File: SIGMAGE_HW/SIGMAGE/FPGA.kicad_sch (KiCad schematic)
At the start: 52 parts, among them J9 TSW10607GS, U41 MMBT2222A, U8 LFE5U25F6BG256I

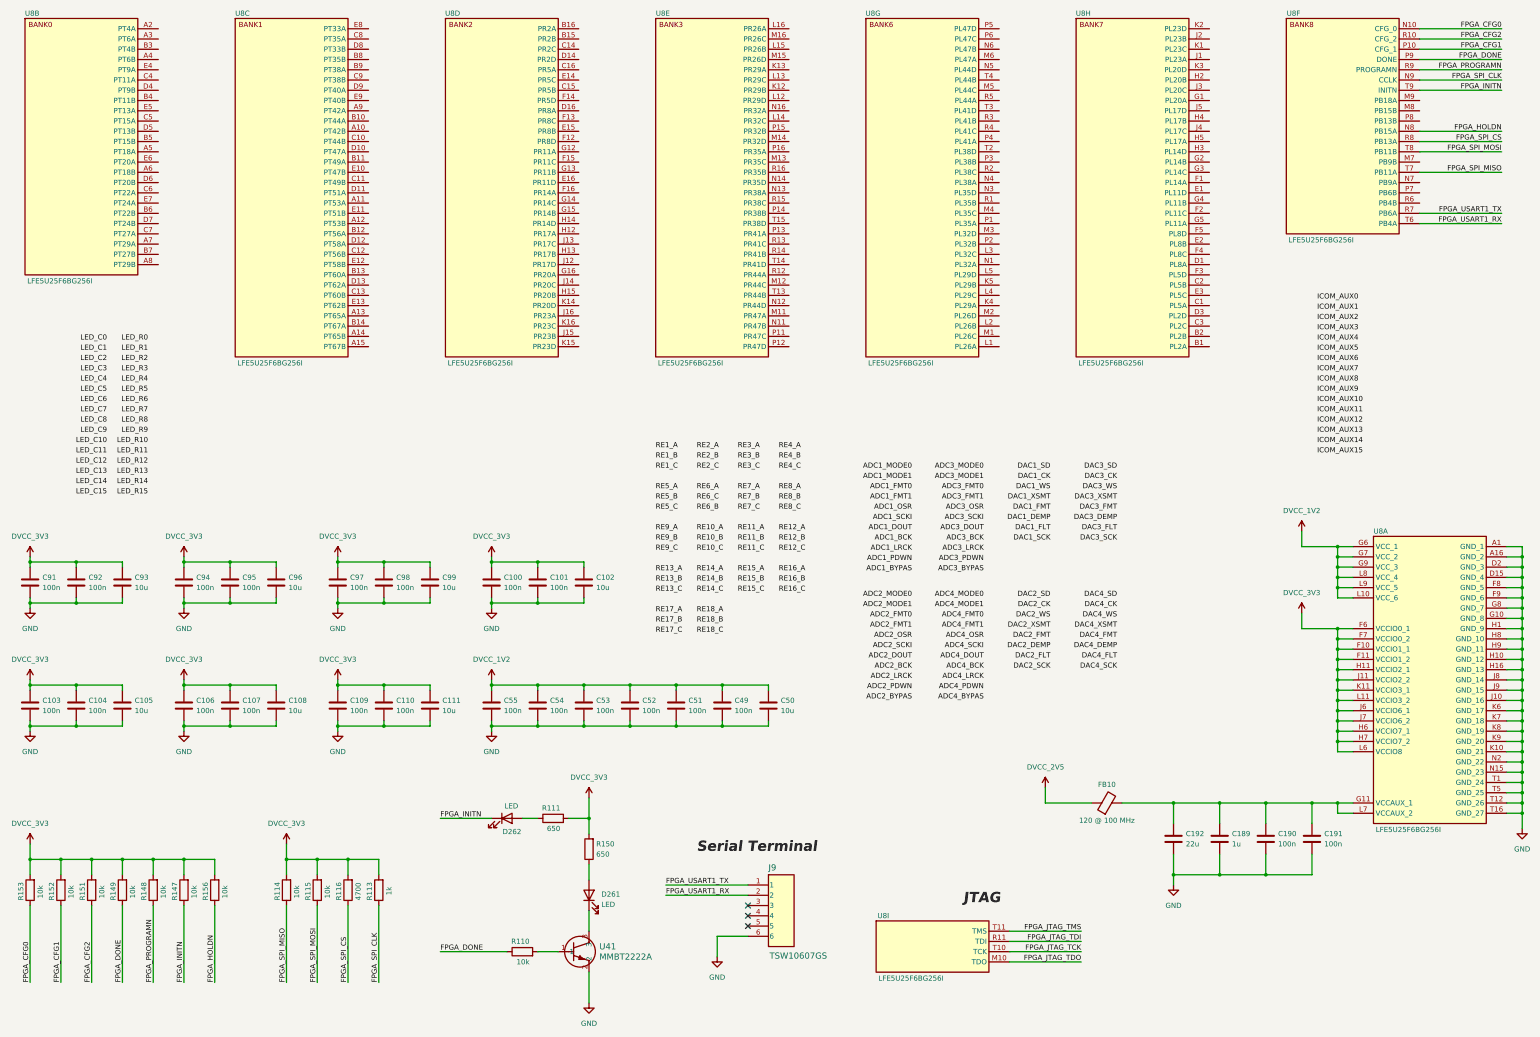
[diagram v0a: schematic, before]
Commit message: changes
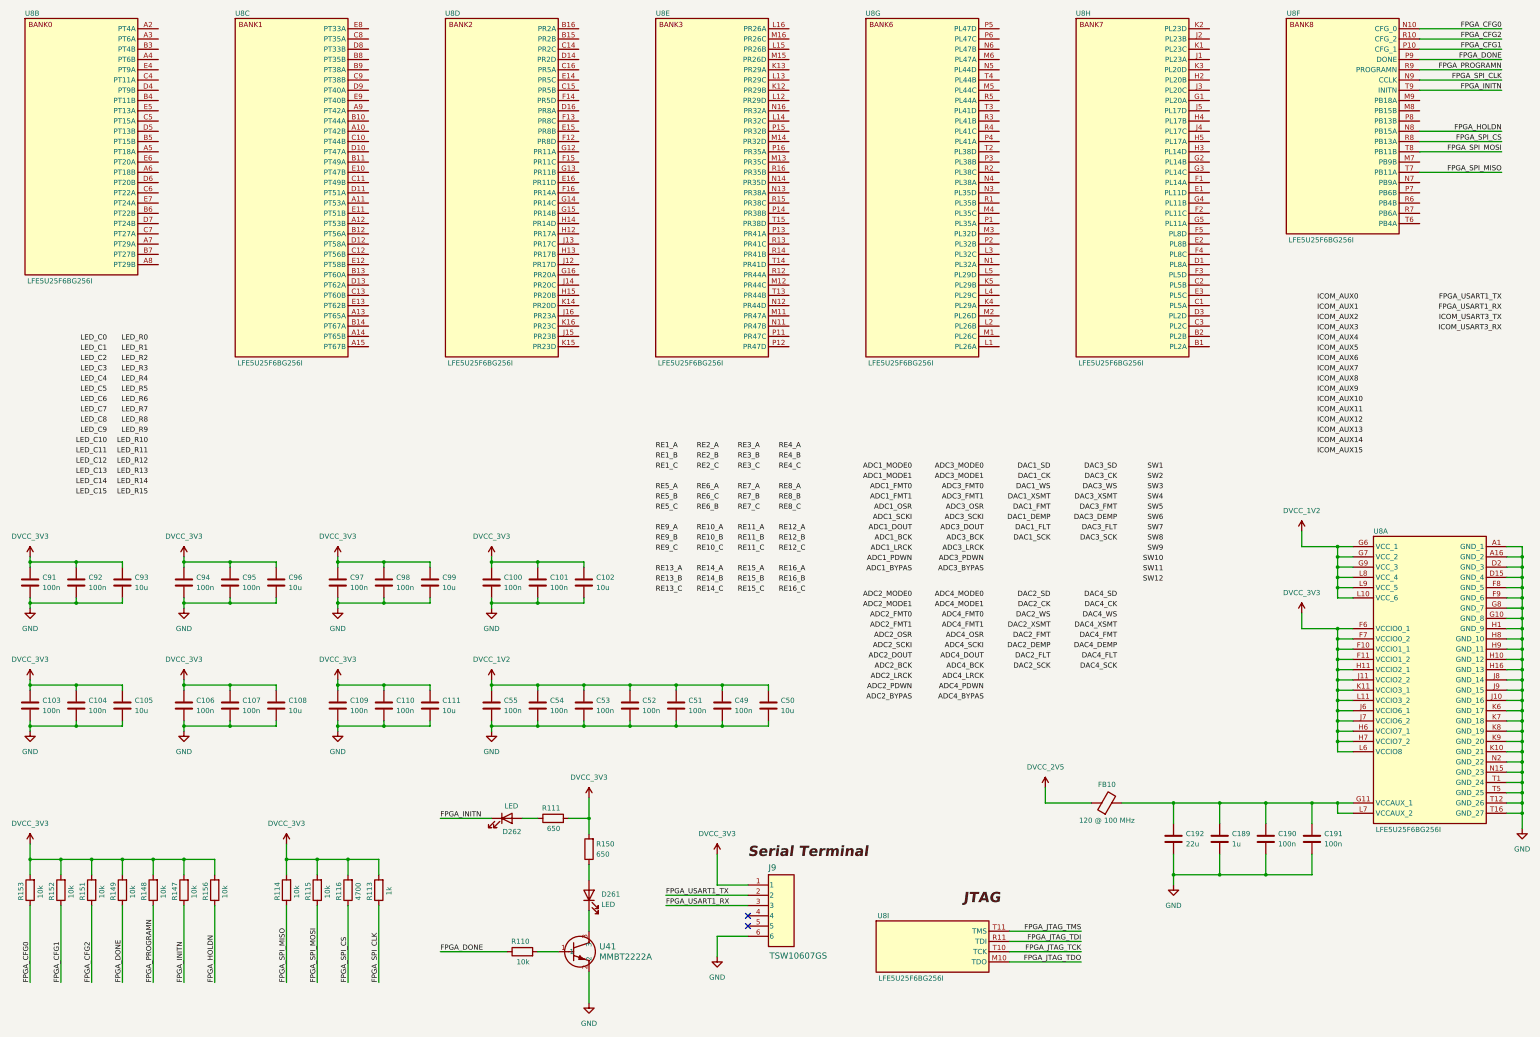
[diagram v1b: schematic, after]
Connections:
- net DVCC_3V3: now also J9.1
- net FPGA_USART1_RX: now also J9.3; no longer J9.2, U8.T6 (PB4A)
- net FPGA_USART1_TX: now also J9.2; no longer J9.1, U8.R7 (PB6A)
- no-connect marks 3 -> 2

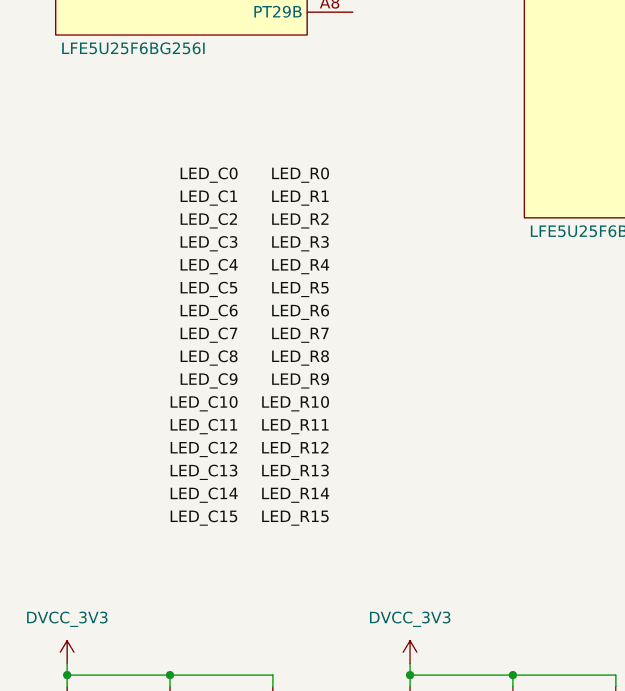
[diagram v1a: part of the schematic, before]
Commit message: before sync sheets
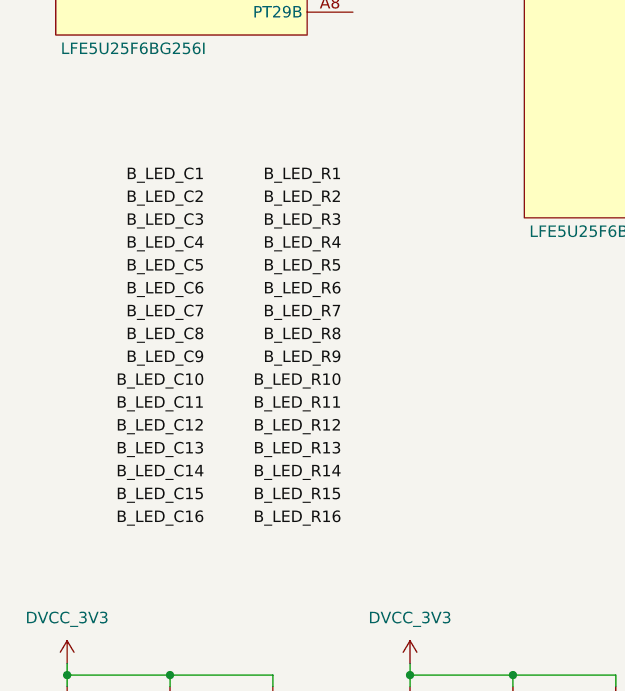
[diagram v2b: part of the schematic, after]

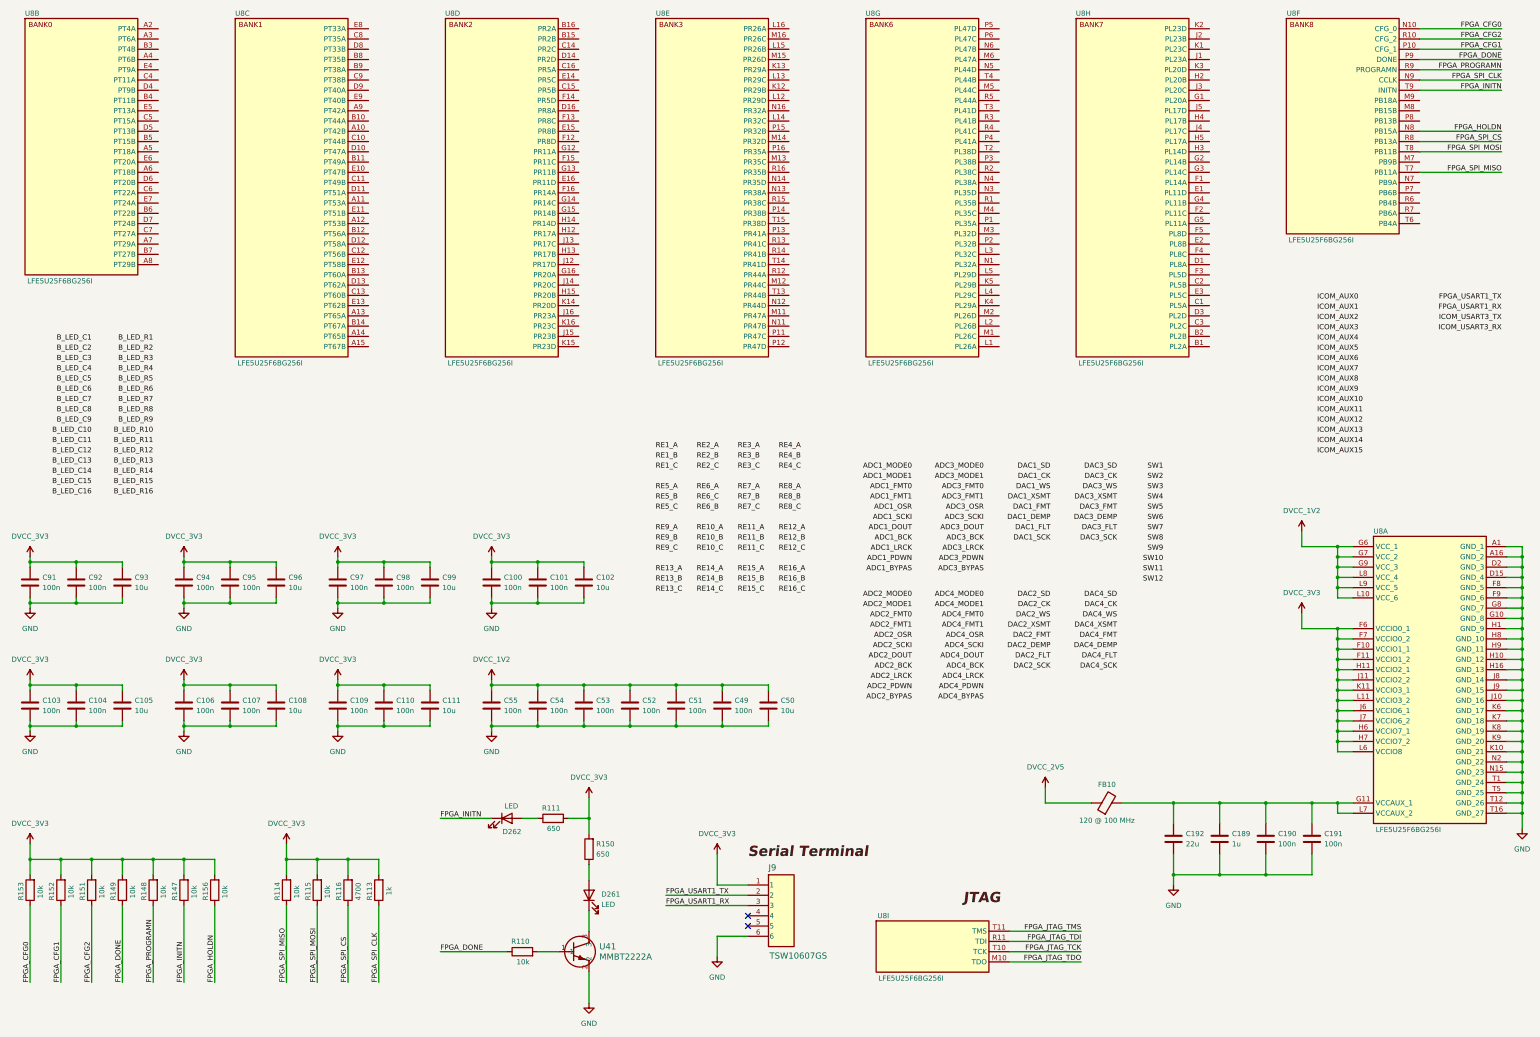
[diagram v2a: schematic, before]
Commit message: finished schematic
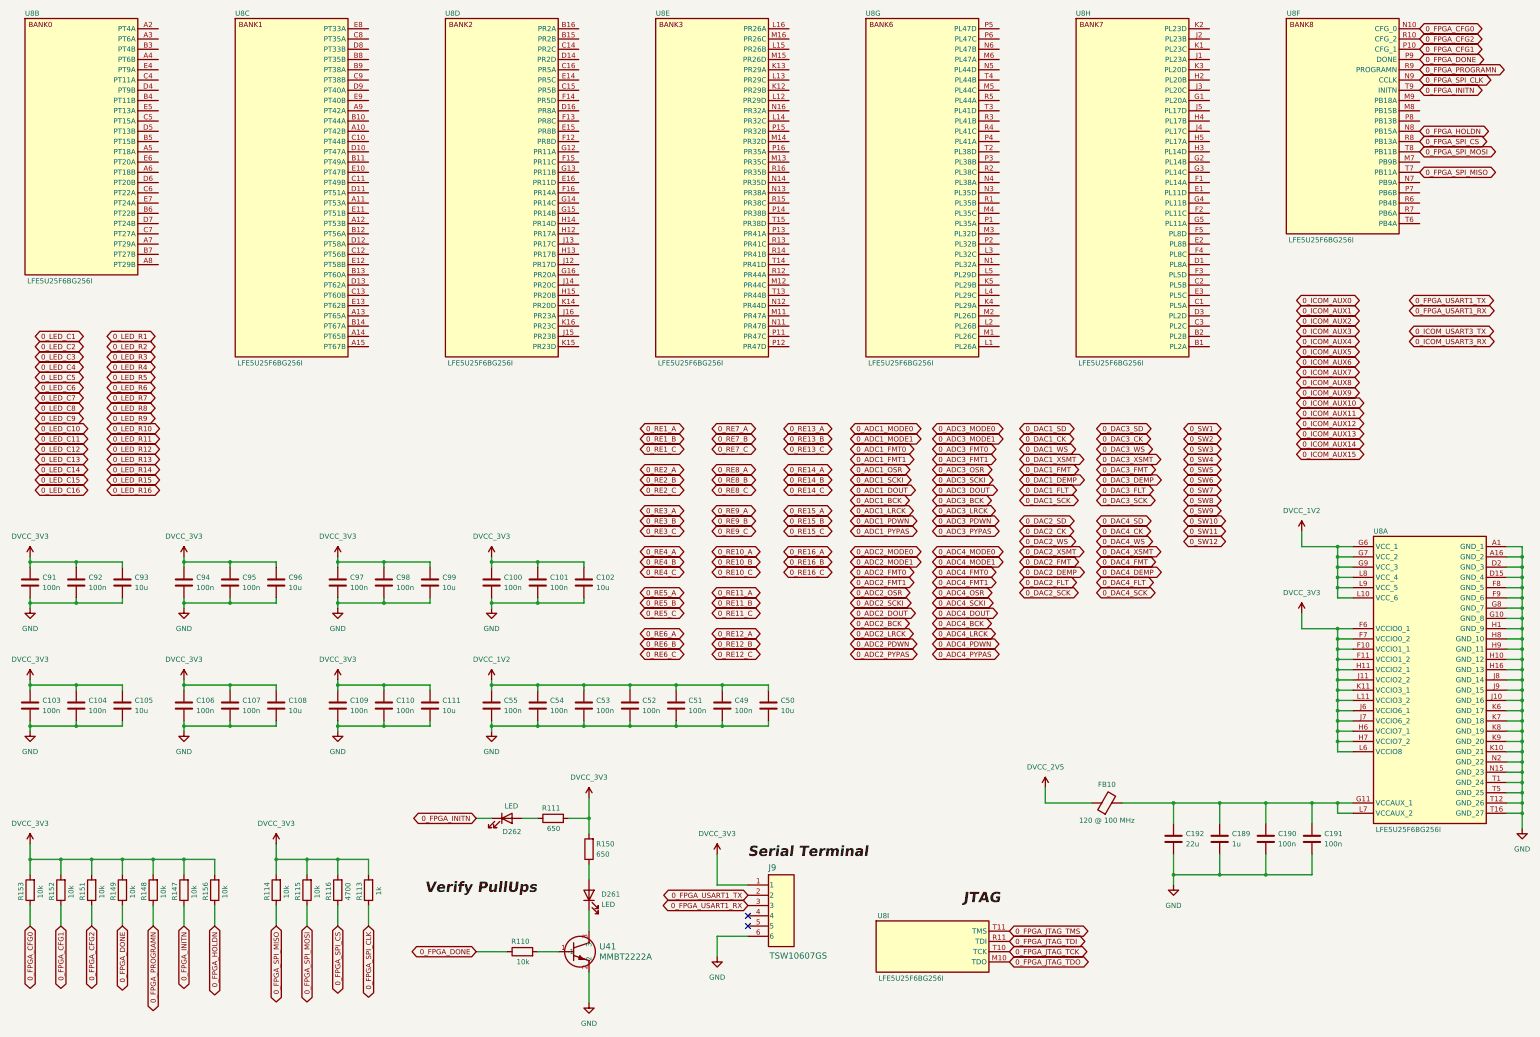
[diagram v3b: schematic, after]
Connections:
- net FPGA_CFG0 renamed 0_FPGA_CFG0
- net FPGA_CFG1 renamed 0_FPGA_CFG1
- net FPGA_CFG2 renamed 0_FPGA_CFG2
- net FPGA_DONE renamed 0_FPGA_DONE
- net FPGA_HOLDN renamed 0_FPGA_HOLDN
- net FPGA_INITN renamed 0_FPGA_INITN
- net FPGA_JTAG_TCK renamed 0_FPGA_JTAG_TCK
- net FPGA_JTAG_TDI renamed 0_FPGA_JTAG_TDI
- net FPGA_JTAG_TDO renamed 0_FPGA_JTAG_TDO
- net FPGA_JTAG_TMS renamed 0_FPGA_JTAG_TMS
- net FPGA_PROGRAMN renamed 0_FPGA_PROGRAMN
- net FPGA_SPI_CLK renamed 0_FPGA_SPI_CLK
- net FPGA_SPI_CS renamed 0_FPGA_SPI_CS
- net FPGA_SPI_MISO renamed 0_FPGA_SPI_MISO
- net FPGA_SPI_MOSI renamed 0_FPGA_SPI_MOSI
- net FPGA_USART1_RX renamed 0_FPGA_USART1_RX
- net FPGA_USART1_TX renamed 0_FPGA_USART1_TX
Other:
- moved on the sheet: R113, R114, R115, R116

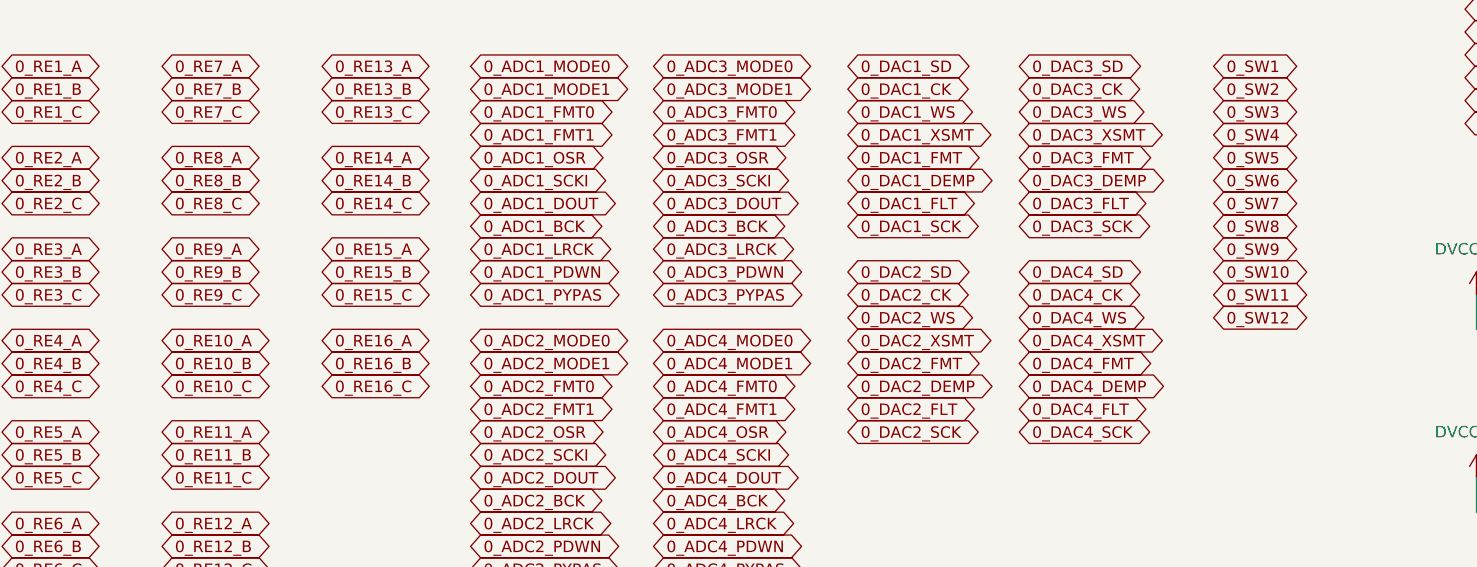
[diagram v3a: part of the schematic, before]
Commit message: uga uga
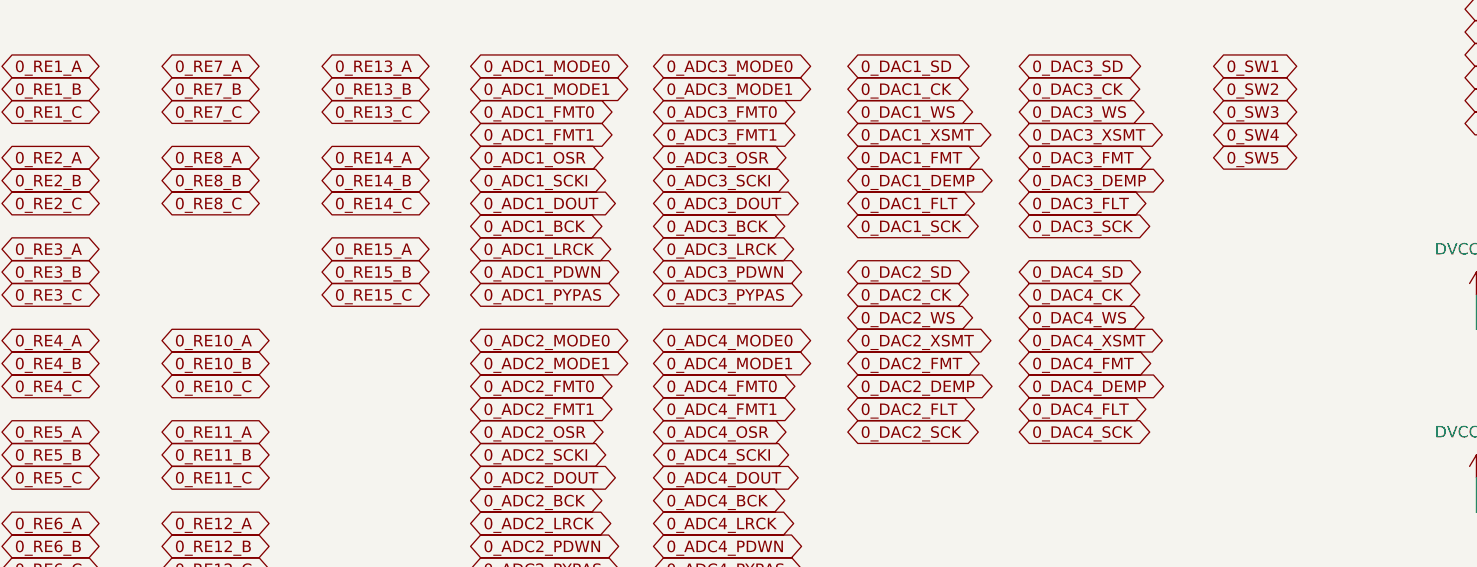
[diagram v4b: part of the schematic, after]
